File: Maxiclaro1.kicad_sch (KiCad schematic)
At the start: 40 parts, among them J1 Screw_Terminal_01x03, J2 ENTRADA, J3 Screw_Terminal_01x03, J4 Screw_Terminal_01x03, J5 Screw_Terminal_01x03, K1 SRD-05VDC-SL-C, K2 SRD-05VDC-SL-C, K3 SRD-05VDC-SL-C, K4 SRD-05VDC-SL-C, Q1 BC547, Q2 BC547, Q3 BC547, Q4 BC547, SW1 SW_DPST_x2, U1 ESP32-DEVKITC-32D, U2 L7805

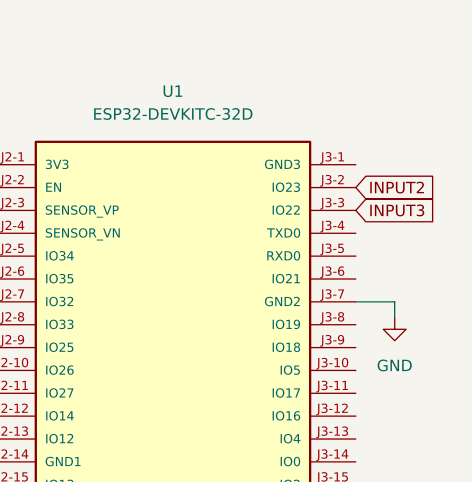
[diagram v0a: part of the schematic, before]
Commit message: Add files via upload
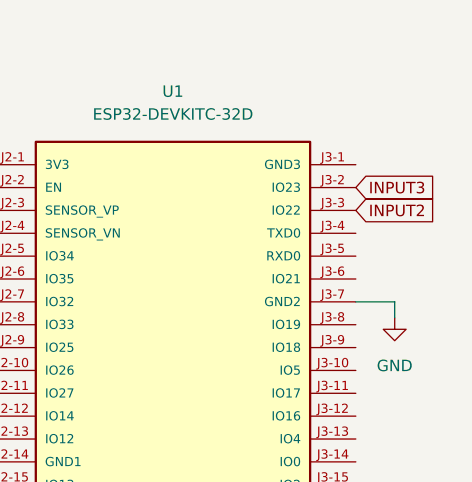
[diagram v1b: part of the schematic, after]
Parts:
- J2: footprint TerminalBlock:TerminalBlock_bornier-2_P5.08mm -> TerminalBlock:TerminalBlock_Altech_AK300-2_P5.00mm
- U2: footprint L7805:TO255P1020X450X2000-3 -> Package_TO_SOT_SMD:TO-263-3_TabPin2
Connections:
- net INPUT2: now also U1.J3-3 (IO22); no longer U1.J3-2 (IO23)
- net INPUT3: now also U1.J3-2 (IO23); no longer U1.J3-3 (IO22)
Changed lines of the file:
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@@
 	(global_label "INPUT3"
 		(shape input)
-		(at 208.28 35.56 0)
+		(at 208.28 33.02 0)
 		(fields_autoplaced yes)
 		(effects
@@
 		)
 		(property "Intersheetrefs" "${INTERSHEET_REFS}"
-			(at 217.9781 35.56 0)
+			(at 217.9781 33.02 0)
 			(show_name yes)
 			(effects
@@
 	(global_label "INPUT2"
 		(shape input)
-		(at 208.28 33.02 0)
+		(at 208.28 35.56 0)
 		(fields_autoplaced yes)
 		(effects
@@
 		)
 		(property "Intersheetrefs" "${INTERSHEET_REFS}"
-			(at 217.9781 33.02 0)
+			(at 217.9781 35.56 0)
 			(show_name yes)
 			(effects
@@
 			)
 		)
-		(property "Footprint" "TerminalBlock:TerminalBlock_bornier-2_P5.08mm"
+		(property "Footprint" "TerminalBlock:TerminalBlock_Altech_AK300-2_P5.00mm"
 			(at 158.75 97.79 0)
 			(effects
@@
 			)
 		)
-		(property "Footprint" "L7805:TO255P1020X450X2000-3"
+		(property "Footprint" "Package_TO_SOT_SMD:TO-263-3_TabPin2"
 			(at 185.293 99.06 0)
 			(effects

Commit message: Add files via upload
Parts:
- SW1: footprint RB141C1100:SW_RB141C1100 -> 2MS1T1B1M2QES:SW_2MS1T1B1M2QES-5
- U2: footprint Package_TO_SOT_SMD:TO-263-3_TabPin2 -> Package_TO_SOT_SMD:TO-263-2
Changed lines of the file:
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@@
 			)
 		)
-		(property "Footprint" "RB141C1100:SW_RB141C1100"
+		(property "Footprint" "2MS1T1B1M2QES:SW_2MS1T1B1M2QES-5"
 			(at 170.18 95.25 0)
 			(effects
@@
 			)
 		)
-		(property "Footprint" "Package_TO_SOT_SMD:TO-263-3_TabPin2"
+		(property "Footprint" "Package_TO_SOT_SMD:TO-263-2"
 			(at 185.293 99.06 0)
 			(effects
